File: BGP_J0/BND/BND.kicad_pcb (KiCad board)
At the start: 2 copper layers, 25 x 28 mm, 7 parts, among them J1 Conn_01x13, J2 Conn_01x03, J3 Conn_01x02, J4 Conn_01x02, J5 Conn_01x03, J6 Conn_01x02, J7 Conn_01x02

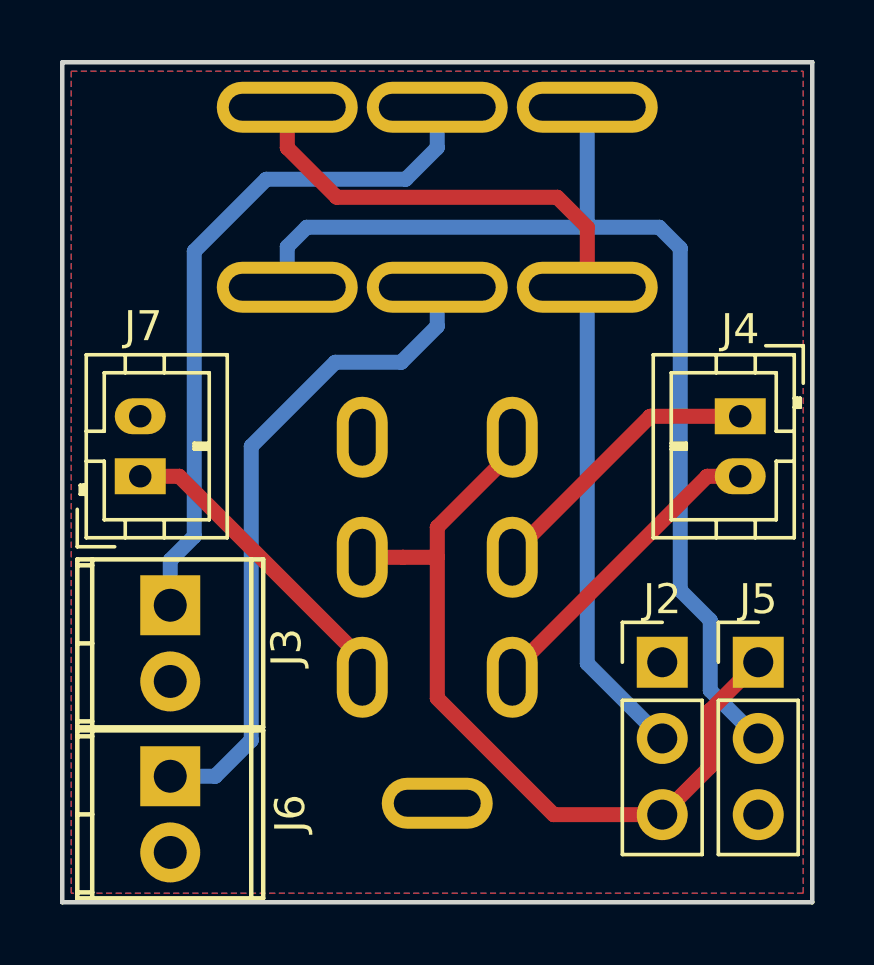
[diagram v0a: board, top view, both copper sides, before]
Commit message: J0 - Panelisation
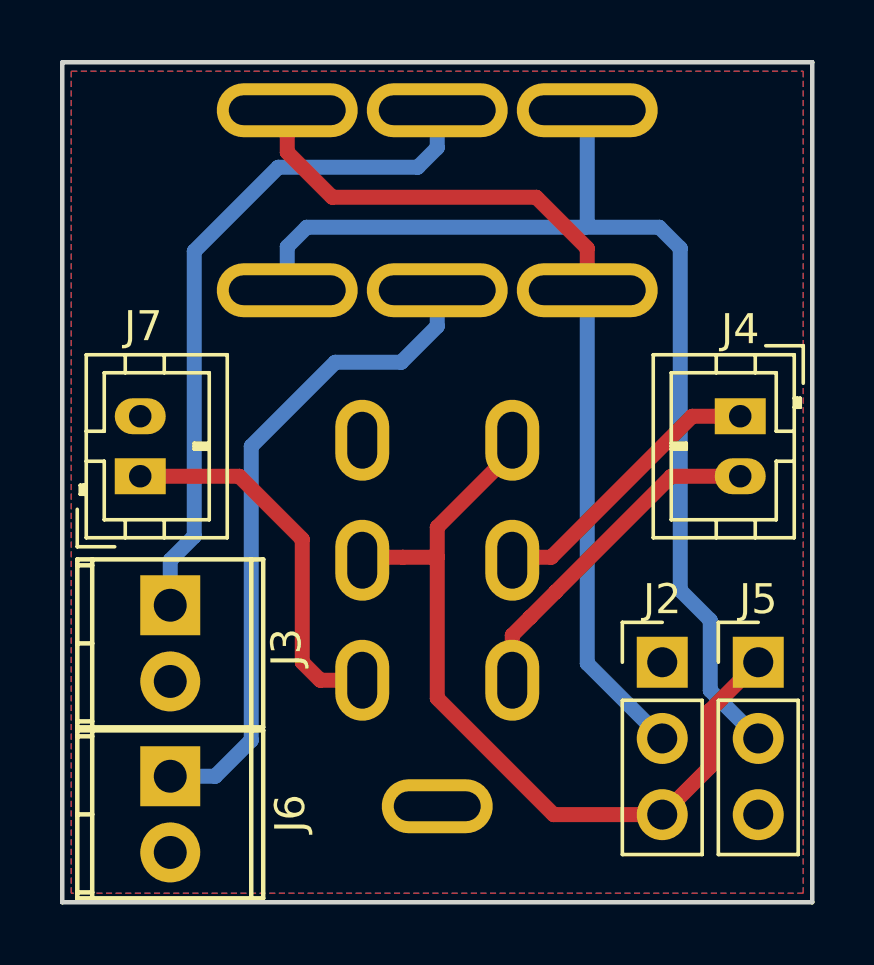
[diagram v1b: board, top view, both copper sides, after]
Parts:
- moved J1 0.10 mm to (112.5, 71.6)
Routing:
- net /BT_O: track 10.5 -> 12.6 mm
- net /V_I: track 10.5 -> 11.2 mm
